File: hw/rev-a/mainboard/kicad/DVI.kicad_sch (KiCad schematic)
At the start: 14 parts, among them J24 NOT_HDMI_A

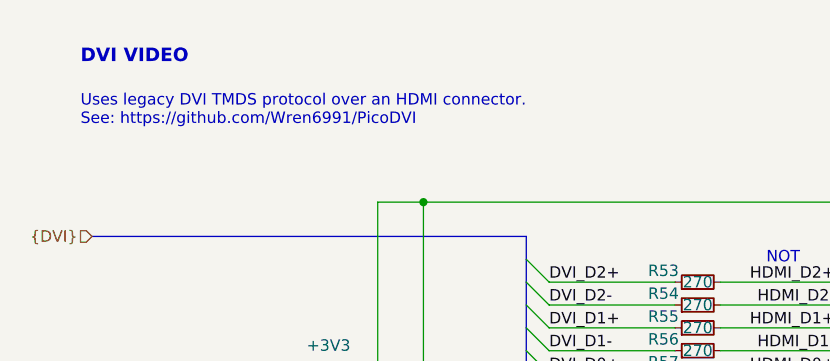
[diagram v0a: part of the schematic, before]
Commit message: hw: tidy schematics for publication
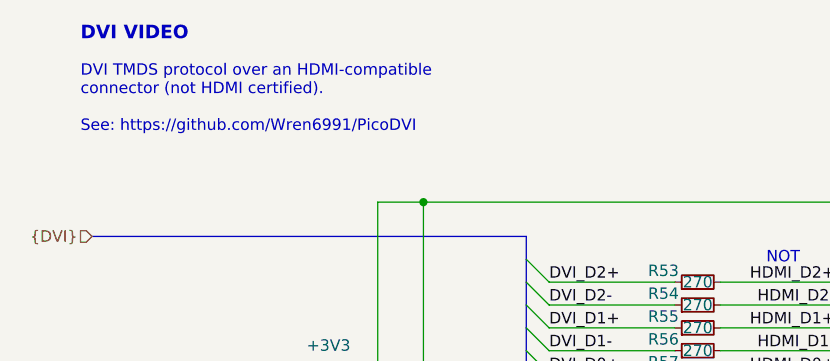
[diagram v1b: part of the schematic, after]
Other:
- note added: "DVI TMDS protocol over an HDMI-compatible connector (not HDMI certified). See: https://github.com/Wren6991/PicoDVI"
- note removed: "Uses legacy DVI TMDS protocol over an HDMI connector. See: https://github.com/Wren6991/PicoDVI"
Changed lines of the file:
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@@
 		)
 	)
-	(text "Uses legacy DVI TMDS protocol over an HDMI connector.\nSee: https://github.com/Wren6991/PicoDVI"
+	(text "DVI TMDS protocol over an HDMI-compatible\nconnector (not HDMI certified).\n\nSee: https://github.com/Wren6991/PicoDVI"
 		(exclude_from_sim no)
-		(at 83.82 50.8 0)
+		(at 83.82 49.53 0)
 		(effects
 			(font
@@
 	(text "DVI VIDEO"
 		(exclude_from_sim no)
-		(at 83.82 45.72 0)
+		(at 83.82 43.18 0)
 		(effects
 			(font
